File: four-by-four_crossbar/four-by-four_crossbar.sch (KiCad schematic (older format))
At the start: 6 parts, among them J1 Conn_02x12_USBC_pins, J2 Conn_02x12_USBC_pins, J3 Conn_02x12_USBC_pins, J4 Conn_02x12_USBC_pins, J5 Conn_02x12_USBC_pins_shielded, J6 Conn_02x12_USBC_pins_shielded

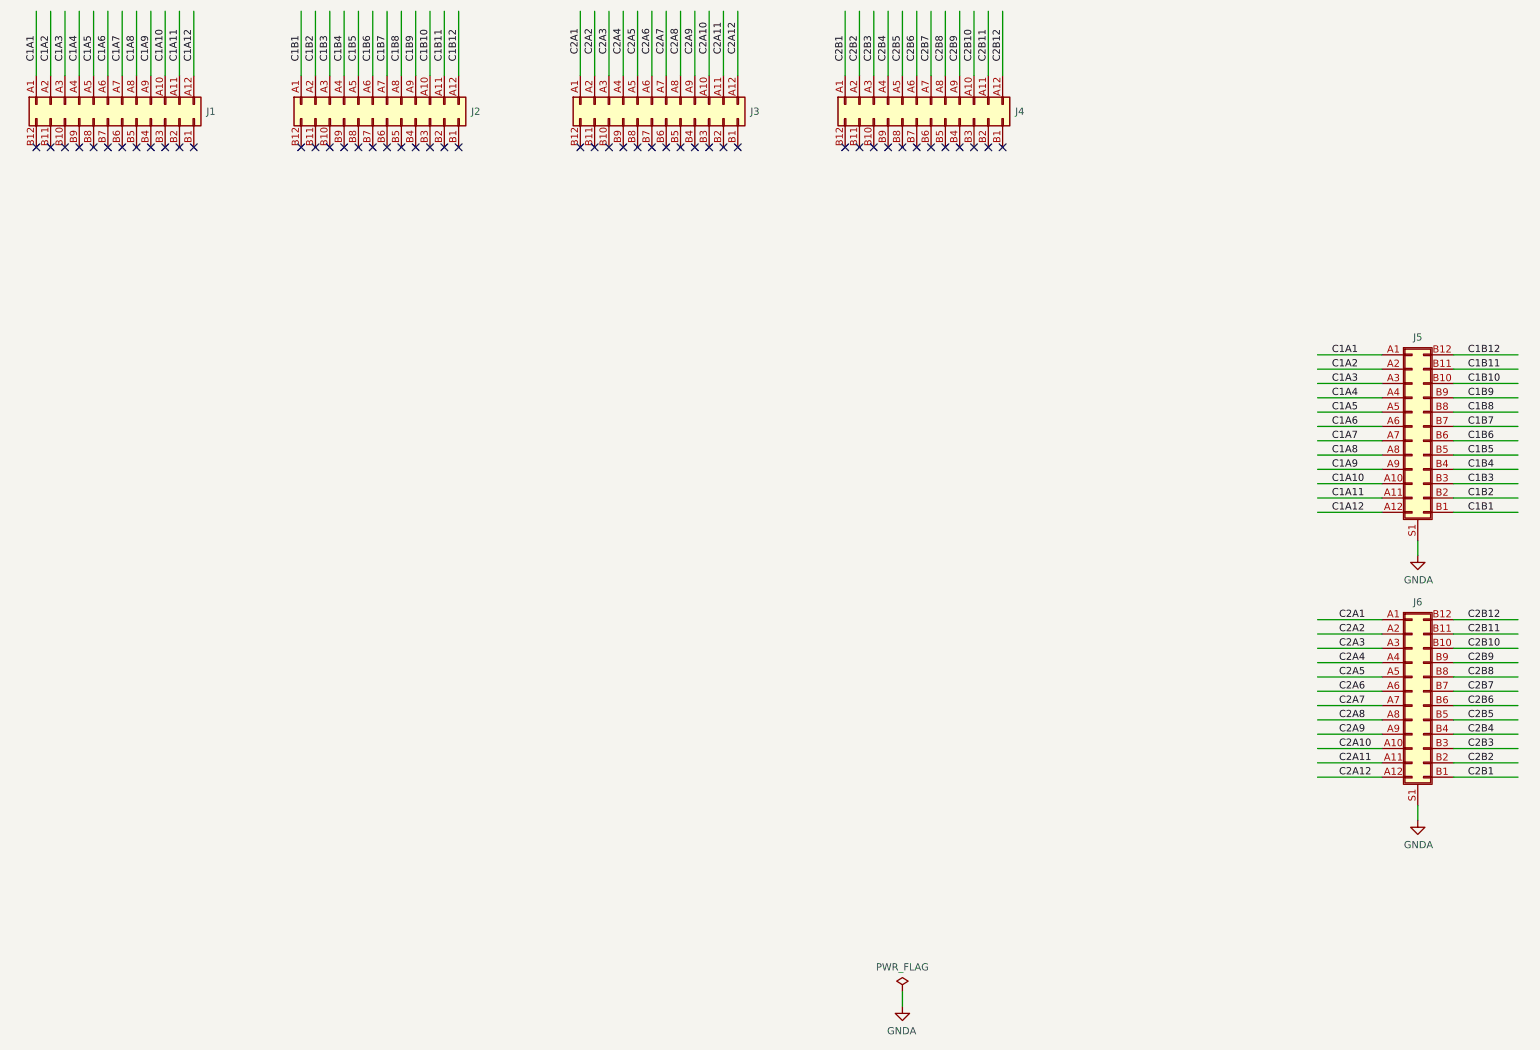
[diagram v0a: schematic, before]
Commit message: take snapshot
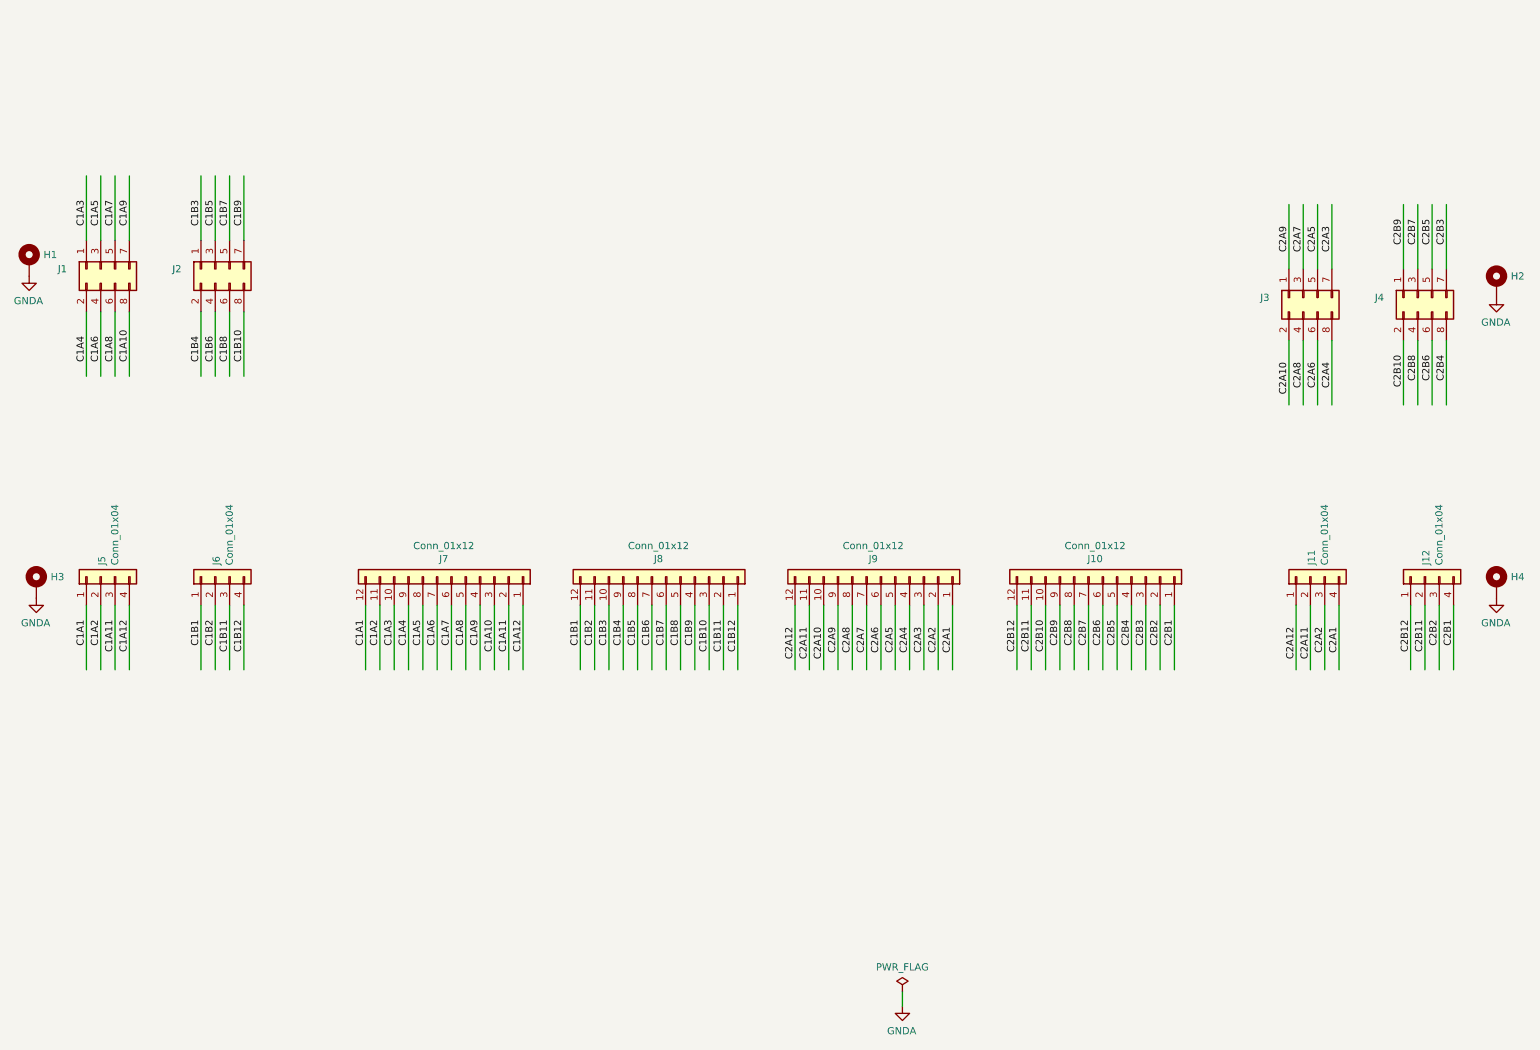
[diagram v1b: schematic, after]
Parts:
- removed J1, J2, J3, J4: Conn_02x12_USBC_pins, my_footprints:PinSocket_2x12_P2.00mm_Vertical_EDGE_USBC_pins, symbol my_syms:Conn_02x12_USBC_pins
- removed J5, J6: Conn_02x12_USBC_pins_shielded, Connector_USB:USB_C_Receptacle_Amphenol_12401548E4-2A, symbol my_syms:Conn_02x12_USBC_pins_shielded
- added H1, H2, H3, H4: MountingHole_Pad, MountingHole:MountingHole_2.2mm_M2_Pad, symbol Mechanical:MountingHole_Pad
- added J1, J2, J3, J4: Conn_02x04_Odd_Even, Connector_PinSocket_2.00mm:PinSocket_2x04_P2.00mm_Vertical_SMD, symbol Connector_Generic:Conn_02x04_Odd_Even
- added J10, J7, J8, J9: Conn_01x12, my_footprints:SAMTEC-MMS-112-02-X-SH-BRIDGE-PAD, symbol Connector_Generic:Conn_01x12
- added J11, J12, J5, J6: Conn_01x04, Connector_PinSocket_2.00mm:PinSocket_1x04_P2.00mm_Vertical_SMD_Pin1Left, symbol Connector_Generic:Conn_01x04
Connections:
- wire segments 99 -> 97
- no-connect marks 48 -> 0
